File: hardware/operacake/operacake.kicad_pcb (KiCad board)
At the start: 4 copper layers, 120 x 75 mm, 152 parts, among them J1 CONN_02X20, J2 CONN_02X20, P1 ADDRESS, P20 GPIO, P22 I2S, P28 SD, P9 BASEBAND, U1 MASWSS0129, U10 74LVC1G58, U11 74LVC1G58, U12 74LVC1G58, U13 74LVC1G58, U14 74AHC1G02, U15 74AHC1G02, U16 74LVC1G19, U2 SKY13322, U3 SKY13322, U4 PCA9557, U5 TC7MBL3245CFT, U6 74LVC1G58, U7 74LVC1G58, U8 74AHC1G08, U9 74AHC1G08

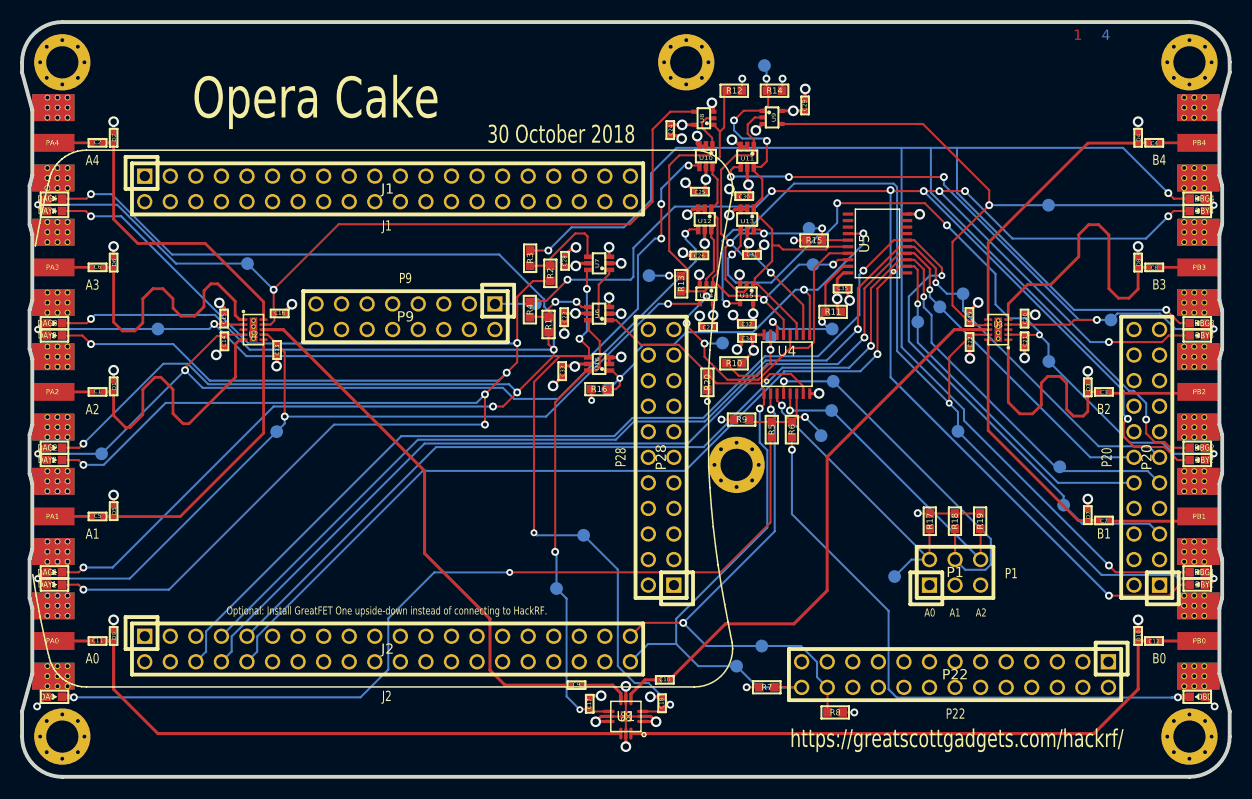
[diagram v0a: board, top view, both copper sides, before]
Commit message: Sync reviewing of hardware
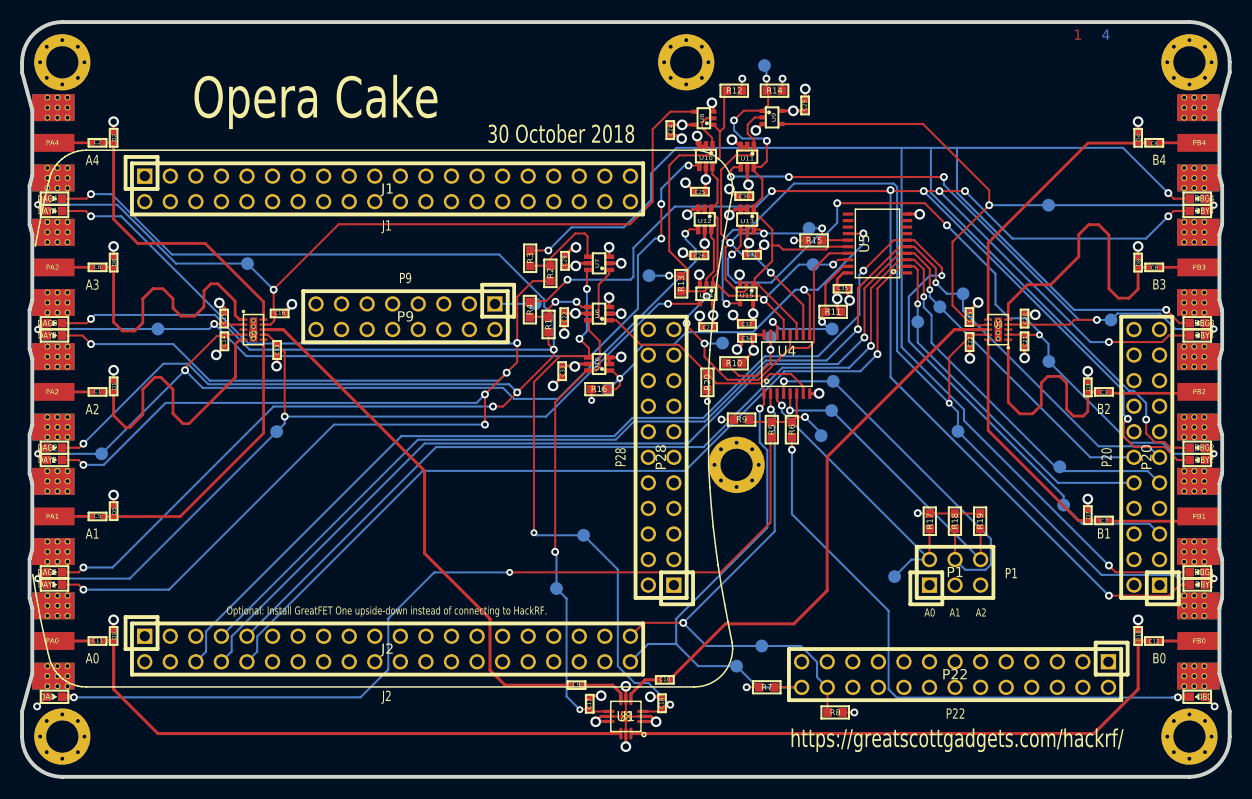
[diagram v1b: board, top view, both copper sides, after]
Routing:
- added copper zone on In1.Cu, net GND
- added copper zone on In2.Cu, net VCC
- removed copper zone on C2, net GND
- removed copper zone on C3, net VCC
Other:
- net class Default removed
